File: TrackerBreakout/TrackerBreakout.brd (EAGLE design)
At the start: 17.8 x 22.9 mm, 15 parts

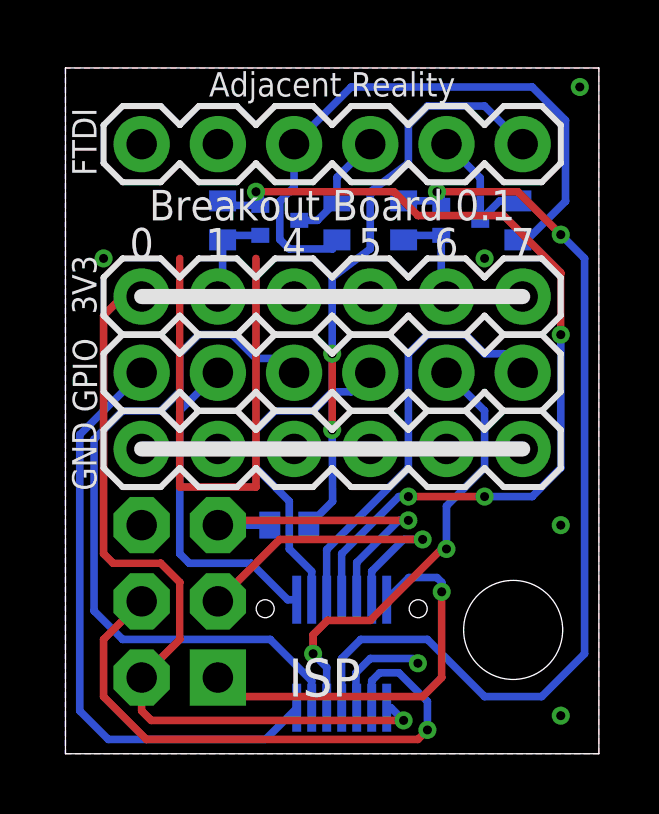
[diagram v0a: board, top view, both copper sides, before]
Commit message: so close
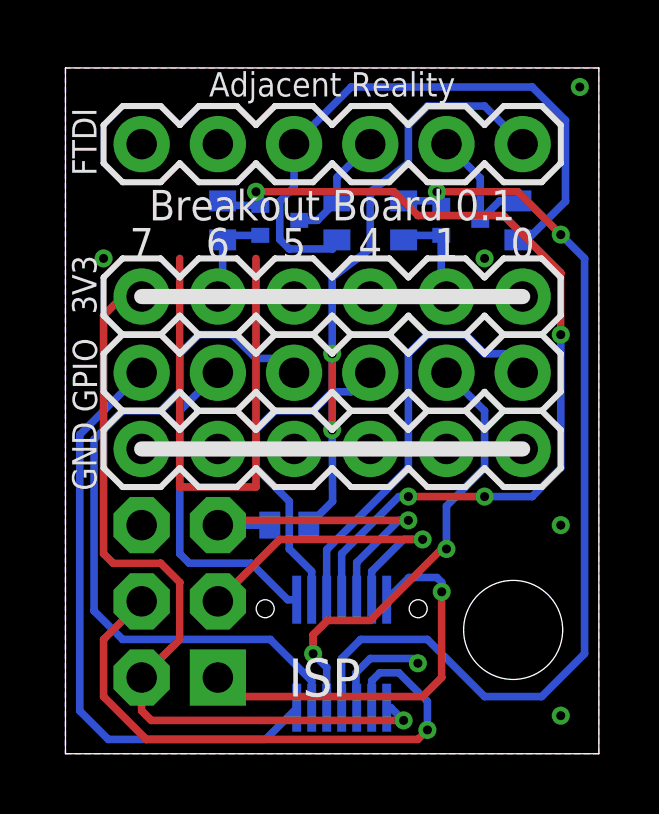
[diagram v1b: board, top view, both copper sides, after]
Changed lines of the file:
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@@
 <wire x1="17.78" y1="22.86" x2="0" y2="22.86" width="0" layer="20"/>
 <wire x1="0" y1="22.86" x2="0" y2="0" width="0" layer="20"/>
-<text x="2.54" y="16.51" size="1.016" layer="21" font="vector" align="bottom-center">0</text>
-<text x="5.08" y="16.51" size="1.016" layer="21" font="vector" align="bottom-center">1</text>
-<text x="7.62" y="16.51" size="1.016" layer="21" font="vector" align="bottom-center">4</text>
-<text x="10.16" y="16.51" size="1.016" layer="21" font="vector" align="bottom-center">5</text>
-<text x="12.7" y="16.51" size="1.016" layer="21" font="vector" align="bottom-center">6</text>
-<text x="15.24" y="16.51" size="1.016" layer="21" font="vector" align="bottom-center">7</text>
+<text x="15.24" y="16.51" size="1.016" layer="21" font="vector" align="bottom-center">0</text>
+<text x="12.7" y="16.51" size="1.016" layer="21" font="vector" align="bottom-center">1</text>
+<text x="10.16" y="16.51" size="1.016" layer="21" font="vector" align="bottom-center">4</text>
+<text x="7.62" y="16.51" size="1.016" layer="21" font="vector" align="bottom-center">5</text>
+<text x="5.08" y="16.51" size="1.016" layer="21" font="vector" align="bottom-center">6</text>
+<text x="2.54" y="16.51" size="1.016" layer="21" font="vector" align="bottom-center">7</text>
 <text x="8.89" y="21.9075" size="0.8128" layer="21" font="vector" align="bottom-center">Adjacent Reality</text>
 <text x="8.89" y="17.78" size="1.016" layer="21" font="vector" align="bottom-center">Breakout Board 0.1</text>
@@
 </signal>
 </signals>
-<errors>
-</errors>
 </board>
 </drawing>
